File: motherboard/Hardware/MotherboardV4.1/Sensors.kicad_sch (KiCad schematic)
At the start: 33 parts, among them J401 0

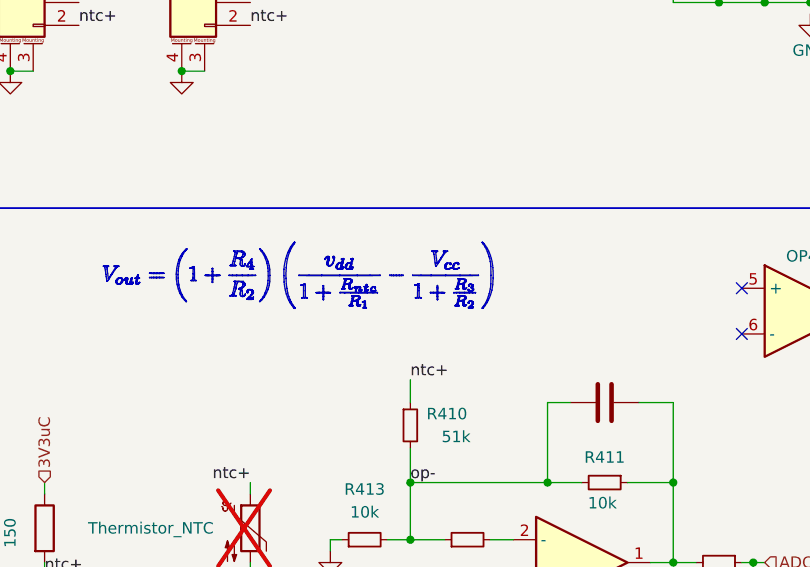
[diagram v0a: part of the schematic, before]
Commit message: changed opamp
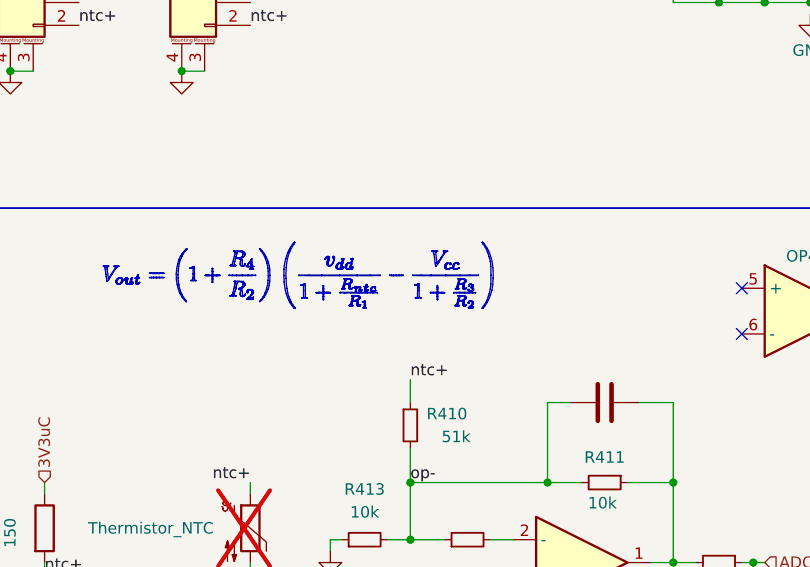
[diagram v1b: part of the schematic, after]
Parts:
- OP401: value TLV9002QDRQ1 -> OPA2377AID
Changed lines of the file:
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@@
 	)
 	(arc
-		(start 90.1269 103.4387)
-		(mid 90.1288 103.4331)
-		(end 90.1339 103.4304)
+		(start 90.1339 103.4304)
+		(mid 90.134 103.4496)
+		(end 90.1269 103.4387)
 		(stroke
 			(width 0.08)
@@
 	)
 	(arc
-		(start 104.2505 108.8744)
-		(mid 104.2414 108.8715)
-		(end 104.24 108.8626)
+		(start 104.24 108.8626)
+		(mid 104.2608 108.8638)
+		(end 104.2505 108.8744)
 		(stroke
 			(width 0.08)
@@
 	)
 	(arc
-		(start 93.9377 106.897)
-		(mid 93.9501 106.9015)
-		(end 93.9446 106.9117)
+		(start 93.9446 106.9117)
+		(mid 93.9291 106.9062)
+		(end 93.9377 106.897)
 		(stroke
 			(width 0.08)
@@
 	)
 	(arc
-		(start 91.2932 107.5106)
-		(mid 91.2925 107.5121)
-		(end 91.2929 107.5181)
+		(start 91.2929 107.5181)
+		(mid 91.2904 107.5149)
+		(end 91.2932 107.5106)
 		(stroke
 			(width 0.08)
@@
 	)
 	(arc
-		(start 103.17 106.7418)
-		(mid 103.1741 106.7445)
-		(end 103.171 106.7481)
+		(start 103.171 106.7481)
+		(mid 103.1705 106.7481)
+		(end 103.17 106.7418)
 		(stroke
 			(width 0.08)
@@
 			)
 		)
-		(property "Value" "TLV9002QDRQ1"
+		(property "Value" "OPA2377AID"
 			(at 155.702 138.684 0)
 			(effects
@@
 			)
 		)
-		(property "Value" "TLV9002QDRQ1"
+		(property "Value" "OPA2377AID"
 			(at 142.24 101.6 0)
 			(effects
@@
 			)
 		)
-		(property "Value" "TLV9002QDRQ1"
+		(property "Value" "OPA2377AID"
 			(at 116.84 144.78 0)
 			(effects
